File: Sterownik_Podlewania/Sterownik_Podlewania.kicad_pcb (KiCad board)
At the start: 2 copper layers, 100 parts, among them J1 Barrel_Jack_MountingPin, J10 Screw_Terminal_01x02, J11 Screw_Terminal_01x02, J12 Screw_Terminal_01x02, J13 Screw_Terminal_01x02, J14 Screw_Terminal_01x02, J15 Screw_Terminal_01x02, J16 Screw_Terminal_01x02, J18 RJ45, J3 RJ45, J4 Conn_01x04_Socket, J5 RJ45, J6 RJ45, J8 RJ45, J9 Screw_Terminal_01x02, K1 SANYOU_SRD_Form_C, K2 SANYOU_SRD_Form_C, K3 SANYOU_SRD_Form_C, K4 SANYOU_SRD_Form_C, K5 SANYOU_SRD_Form_C, Q1 BC547, Q2 BC547, Q3 BC547, Q4 BC547, Q5 BC547, SW1 SW_Nidec_CAS-120A1, SW2 SW_Nidec_CAS-120A1, SW3 SW_Nidec_CAS-120A1, SW4 SW_Nidec_CAS-120A1, SW5 SW_Nidec_CAS-120A1, SW6 SW_Nidec_CAS-120A1, SW8 SW_Nidec_CAS-120A1, U1 ESP32-DEVKITC, U2 HHG1D-1, U3 L7805, U4 LD1117S33TR_SOT223, U5 757

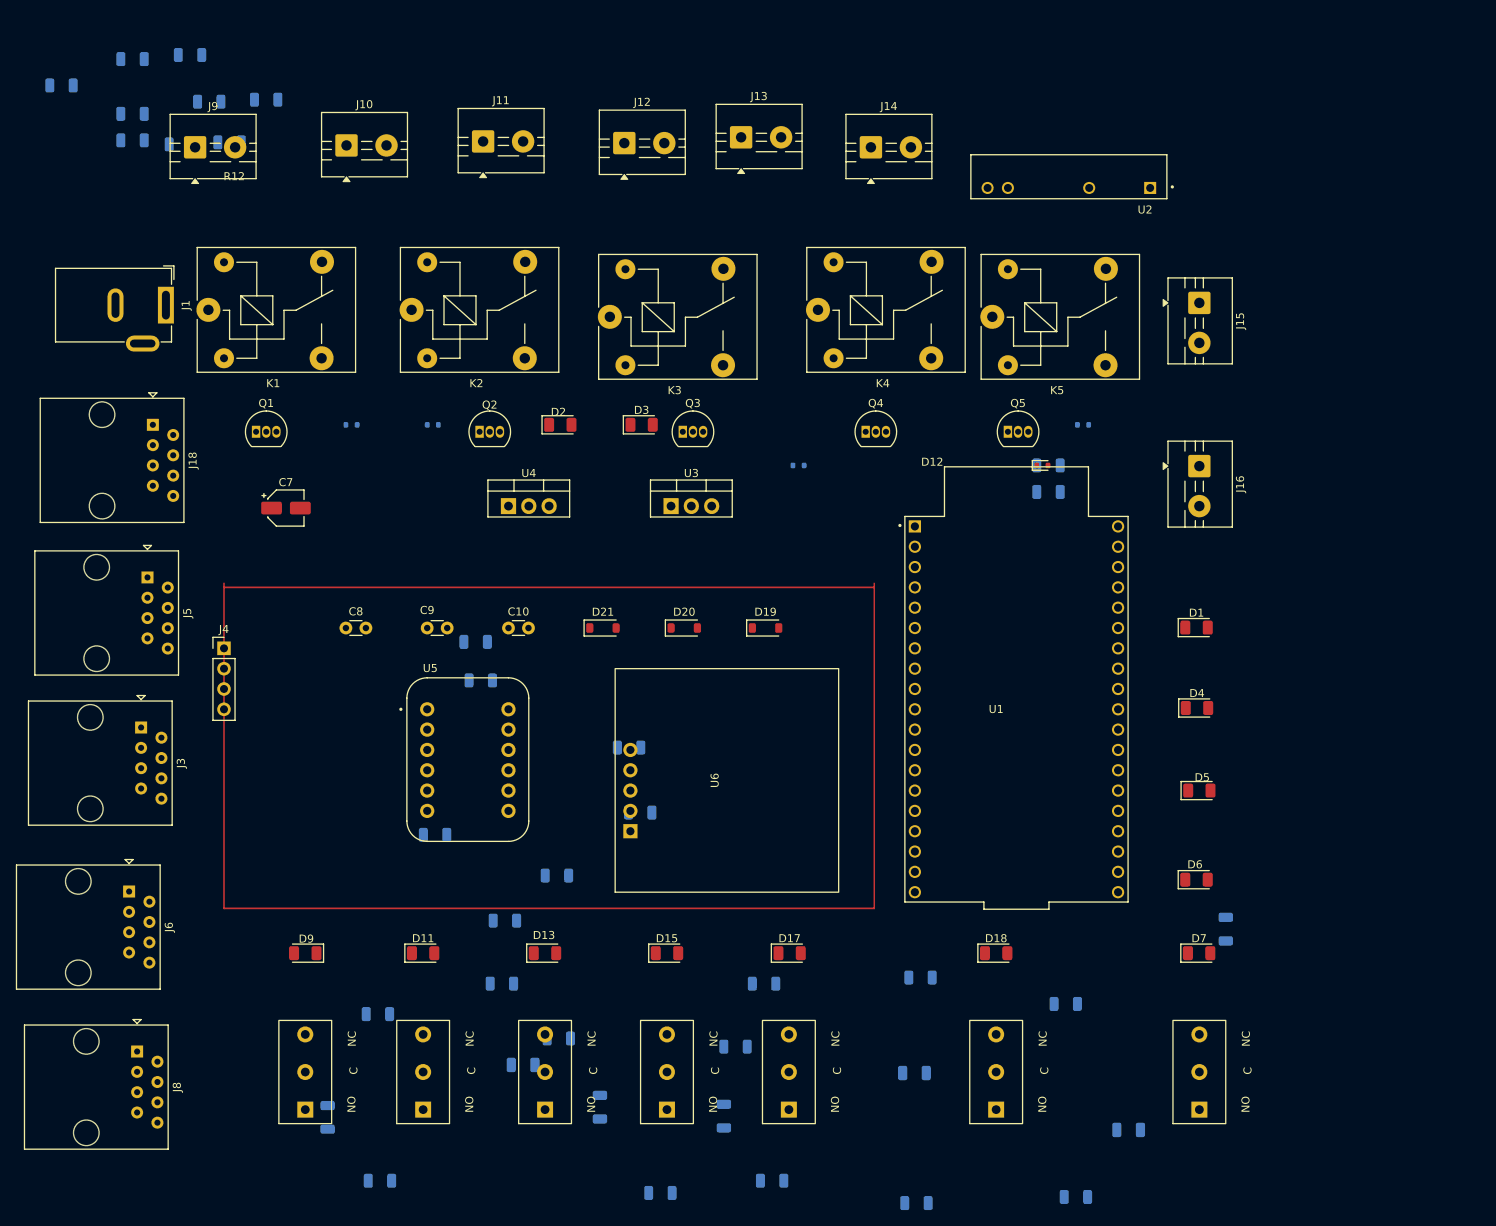
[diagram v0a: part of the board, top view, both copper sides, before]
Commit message: Wstępny finalny rozkład płytki, narysowanie outlinu
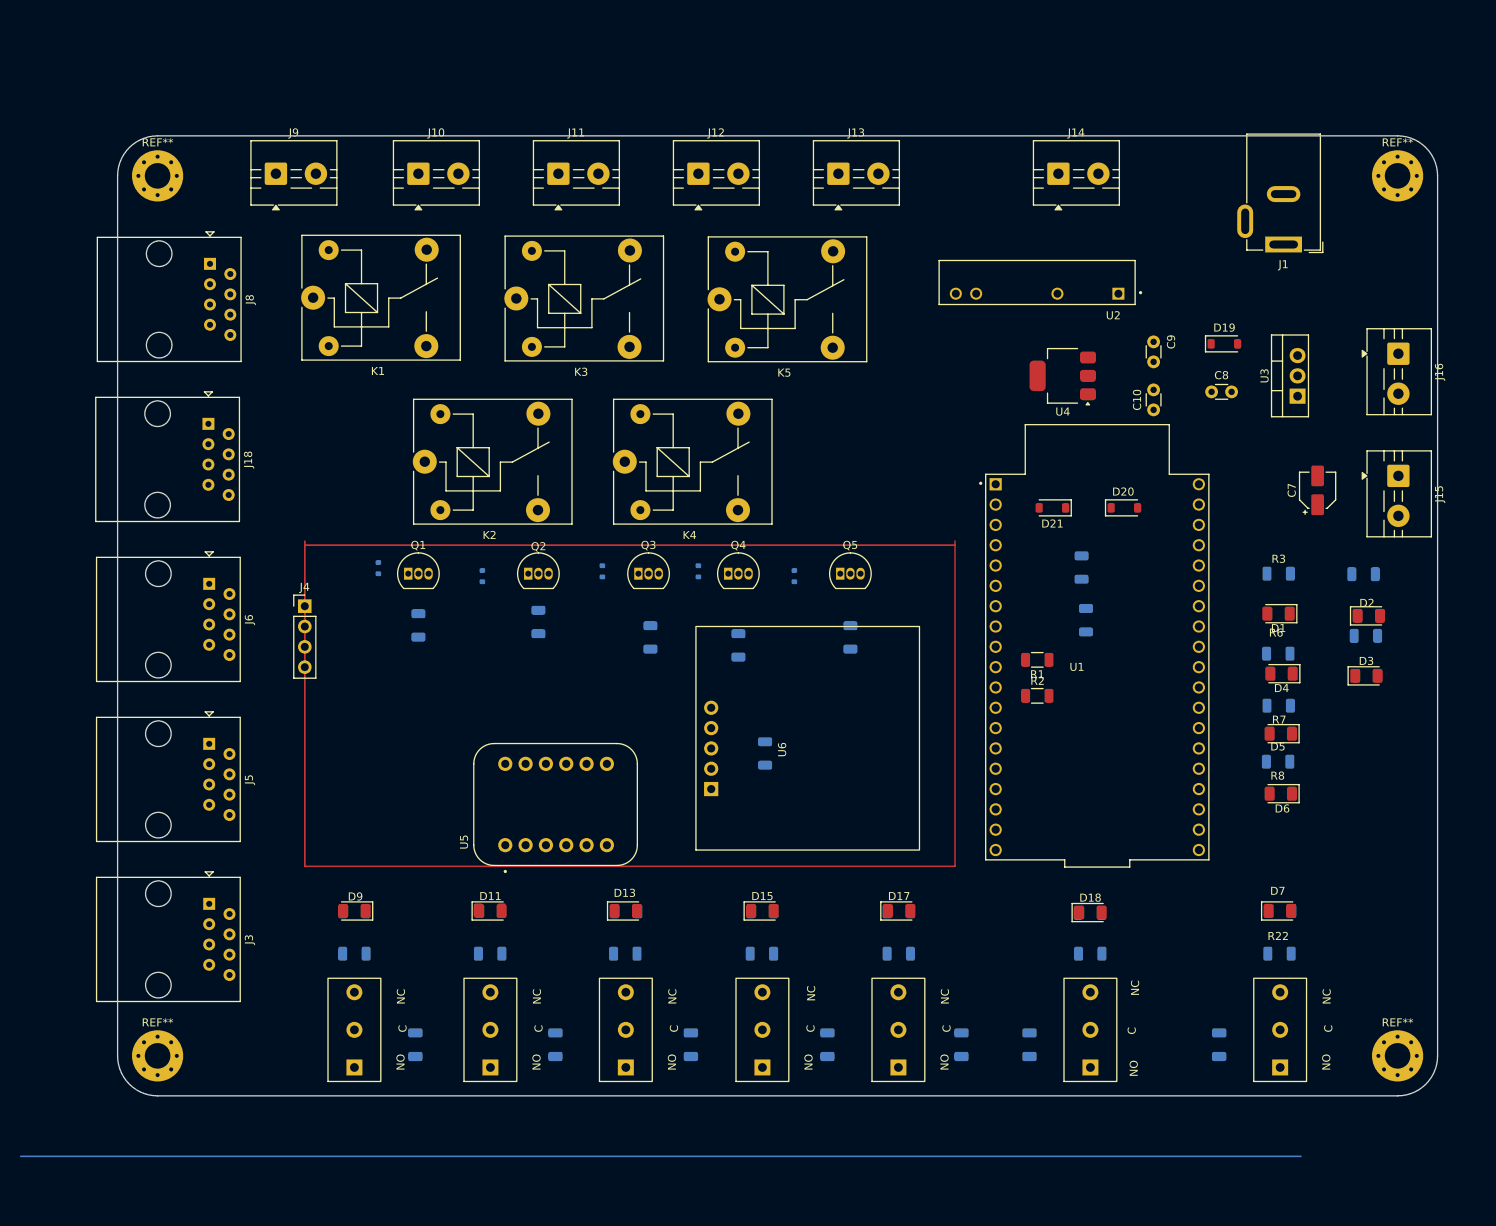
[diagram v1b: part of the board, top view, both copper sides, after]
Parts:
- added REF**: MountingHole_3.2mm_M3_Pad_Via, MountingHole:MountingHole_3.2mm_M3_Pad_Via, F.Cu at (197.5, 150.0)
- added REF**: MountingHole_3.2mm_M3_Pad_Via, MountingHole:MountingHole_3.2mm_M3_Pad_Via, F.Cu at (42.5, 40.0)
- added REF**: MountingHole_3.2mm_M3_Pad_Via, MountingHole:MountingHole_3.2mm_M3_Pad_Via, F.Cu at (42.5, 150.0)
- added REF**: MountingHole_3.2mm_M3_Pad_Via, MountingHole:MountingHole_3.2mm_M3_Pad_Via, F.Cu at (197.5, 40.0)
- D12: moved to B.Cu
- R1, R2: moved to F.Cu
- U4: footprint Package_TO_SOT_THT:TO-220-3_Vertical -> Package_TO_SOT_SMD:SOT-223
- moved R5 166.1 mm to (193.5, 97.5)
- moved R4 164.3 mm to (193.2, 89.8)
- moved R2 143.9 mm to (152.5, 105.0), turned to 0 degrees
- moved J1 139.9 mm to (183.2, 48.6), turned to 180 degrees
- moved R1 135.8 mm to (152.5, 100.5)
- moved C7 129.0 mm to (187.5, 79.3), turned to 90 degrees
- moved R10 113.1 mm to (118.4, 112.2), turned to 90 degrees
- moved C8 112.2 mm to (174.2, 67.0)
- moved R22 106.6 mm to (182.7, 137.2)
- moved D2 103.8 mm to (193.9, 95.0)
- moved R3 100.7 mm to (182.6, 89.7)
- moved R6 99.8 mm to (182.6, 99.7)
- moved R19 99.2 mm to (129.1, 97.7), turned to 90 degrees
- moved J8 98.9 mm to (49.0, 51.0)
- moved C9 97.6 mm to (167.0, 60.8), turned to -90 degrees
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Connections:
- U1 pad 15: /WIFI -> /SEN0193_WYJŚCIE
- U1 pad 23: /SEN0193_WYJŚCIE -> /TRYB
- U1 pad 24: /TRYB -> /WIFI
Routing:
- net (no net): track 0.00 -> 160.0 mm
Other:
- board outline added: 165 x 120 mm
